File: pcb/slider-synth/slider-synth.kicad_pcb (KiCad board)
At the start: 2 copper layers, 100 x 80.6 mm, 51 parts, among them J1 USB4105, J2 PJ-325C5-G, J3 Conn_01x01_Pin, J4 Conn_01x01_Pin, SW1 SW_SPST, SW2 SW_SPST, SW3 RotaryEncoder_Switch, U1 ESP32-S3-WROOM-2, U2 LM3940IMPX-3.3/NOPB, U32 MCP4922, U33 LM386, U34 LM386

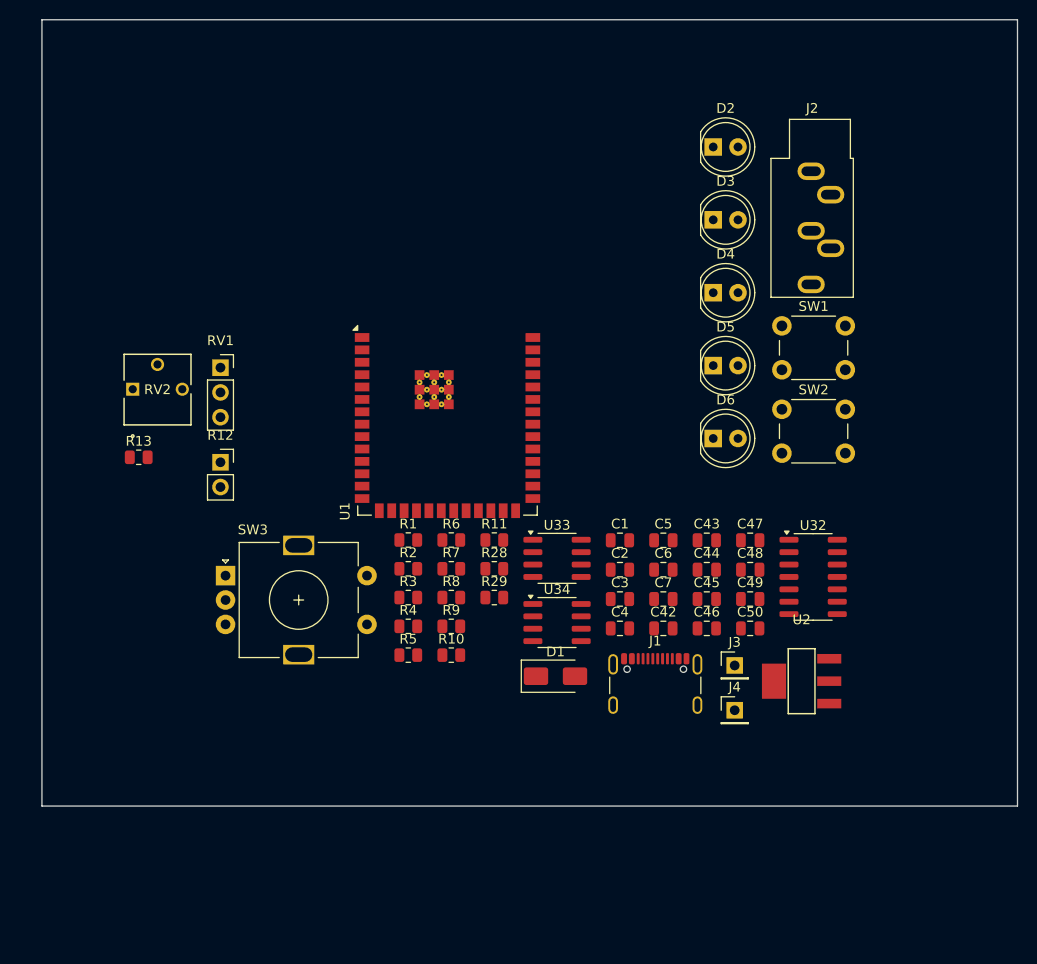
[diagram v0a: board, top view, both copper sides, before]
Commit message: footprints and routing
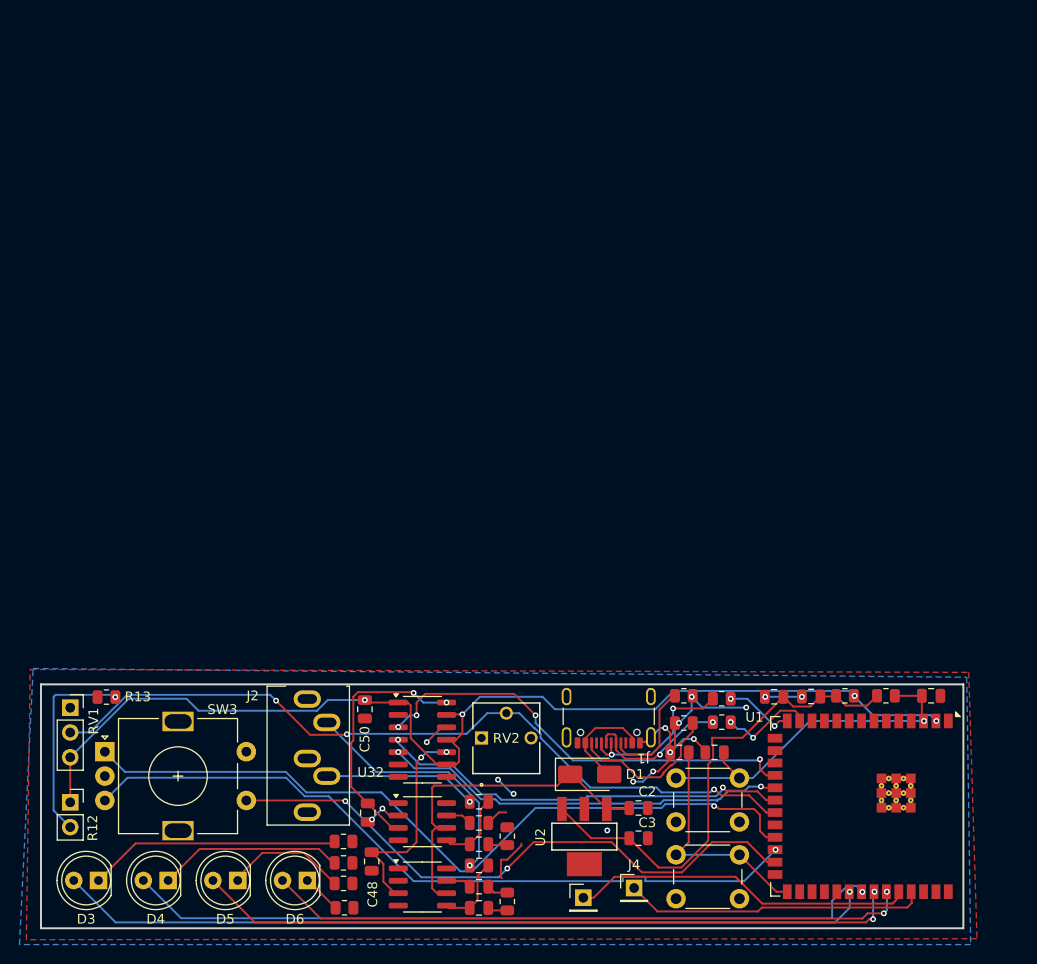
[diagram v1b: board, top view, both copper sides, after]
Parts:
- removed D2: LED, LED_THT:LED_D5.0mm
- removed R7: 330Ω, Resistor_SMD:R_0805_2012Metric
- moved D3 92.5 mm to (106.4, 131.9), turned to 180 degrees
- moved D4 82.2 mm to (113.5, 131.9), turned to 180 degrees
- moved J2 74.8 mm to (127.8, 113.3)
- moved D5 71.8 mm to (120.7, 131.9), turned to 180 degrees
- moved U1 62.9 mm to (188.2, 124.3), turned to -90 degrees
- moved D6 61.5 mm to (127.8, 131.9), turned to 180 degrees
- moved RV2 50.6 mm to (145.7, 117.3)
- moved R3 50.0 mm to (187.1, 113.0)
- moved C48 49.0 mm to (134.4, 130.0), turned to 90 degrees
- moved SW1 47.6 mm to (165.6, 121.4)
- moved SW2 46.9 mm to (165.6, 129.3)
- moved R4 45.3 mm to (182.9, 113.0)
- moved C47 45.1 mm to (145.4, 132.6)
- moved C49 44.9 mm to (134.0, 125.0), turned to 90 degrees
- moved U32 43.4 mm to (139.6, 117.5)
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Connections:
- U1 pad 10: LED4 -> unconnected-(U1-IO17-Pad10)
- U1 pad 15: RotA -> unconnected-(U1-IO3-Pad15)
- U1 pad 22: LED1 -> unconnected-(U1-IO14-Pad22)
- U1 pad 23: unconnected-(U1-IO21-Pad23) -> RotA
- U1 pad 24: unconnected-(U1-IO47-Pad24) -> RotB
- U1 pad 25: unconnected-(U1-IO48-Pad25) -> RotSw
- U1 pad 32: unconnected-(U1-MTCK/IO39-Pad32) -> LED1
- U1 pad 33: unconnected-(U1-MTDO/IO40-Pad33) -> LED2
- U1 pad 34: unconnected-(U1-MTDI/IO41-Pad34) -> LED3
- U1 pad 35: unconnected-(U1-MTMS/IO42-Pad35) -> LED4
- U1 pad 4: RotB -> unconnected-(U1-IO4-Pad4)
- U1 pad 5: RotSw -> unconnected-(U1-IO5-Pad5)
- U1 pad 8: LED2 -> unconnected-(U1-IO15-Pad8)
- U1 pad 9: LED3 -> unconnected-(U1-IO16-Pad9)
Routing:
- net VDD: track 0.00 -> 113.3 mm, vias 0 -> 4
- net LED1: track 0.00 -> 83.6 mm, vias 0 -> 1
- net LinearPot: track 0.00 -> 81.2 mm, vias 0 -> 3
- net RotA: track 0.00 -> 79.1 mm, vias 0 -> 1
- net LED2: track 0.00 -> 78.0 mm, vias 0 -> 1
- net RotB: track 0.00 -> 76.3 mm, vias 0 -> 1
- net LED3: track 0.00 -> 72.5 mm, vias 0 -> 2
- net LED4: track 0.00 -> 65.8 mm, vias 0 -> 2
- net RotSw: track 0.00 -> 62.4 mm, vias 0 -> 2
- net GND: track 0.00 -> 51.2 mm, vias 0 -> 16
- net 3v3: track 0.00 -> 49.8 mm
- net CS: track 0.00 -> 45.5 mm, vias 0 -> 4
- net SCK: track 0.00 -> 42.6 mm, vias 0 -> 2
- net SDI: track 0.00 -> 41.7 mm, vias 0 -> 2
- net 5v: track 0.00 -> 37.0 mm
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- added copper zone on B.Cu, net GND
- added copper zone on F.Cu, net GND
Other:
- board size 100 x 80.6 mm -> 94.6 x 25 mm
